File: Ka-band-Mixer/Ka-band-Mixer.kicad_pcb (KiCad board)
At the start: 4 copper layers, 58.9 x 41.9 mm, 75 parts, among them J1 Conn_01x02_Male, J2 Conn_01x02_Male, J3 Connector_Conn_01x02_Male, J4 Conn_01x05_Male, J5 SMA_END-frequencySintesizer, U1 ADF4150HV, U2 LT1962-3.3, U3 LT3010, U4 HMC739LP4E, U5 LT1962-5, U6 LT1962-5, U7 HMC292ALC3B, X1 IQXT-220-1

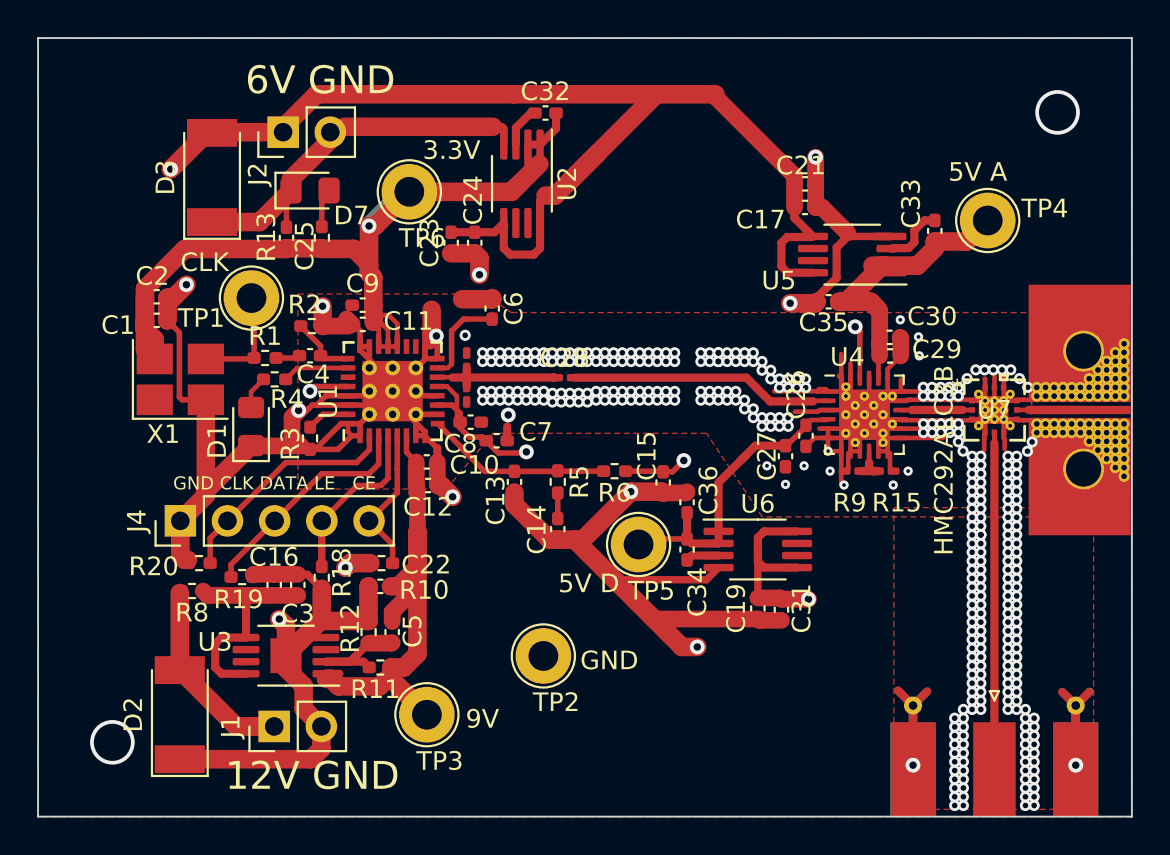
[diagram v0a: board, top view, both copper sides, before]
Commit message: update bom
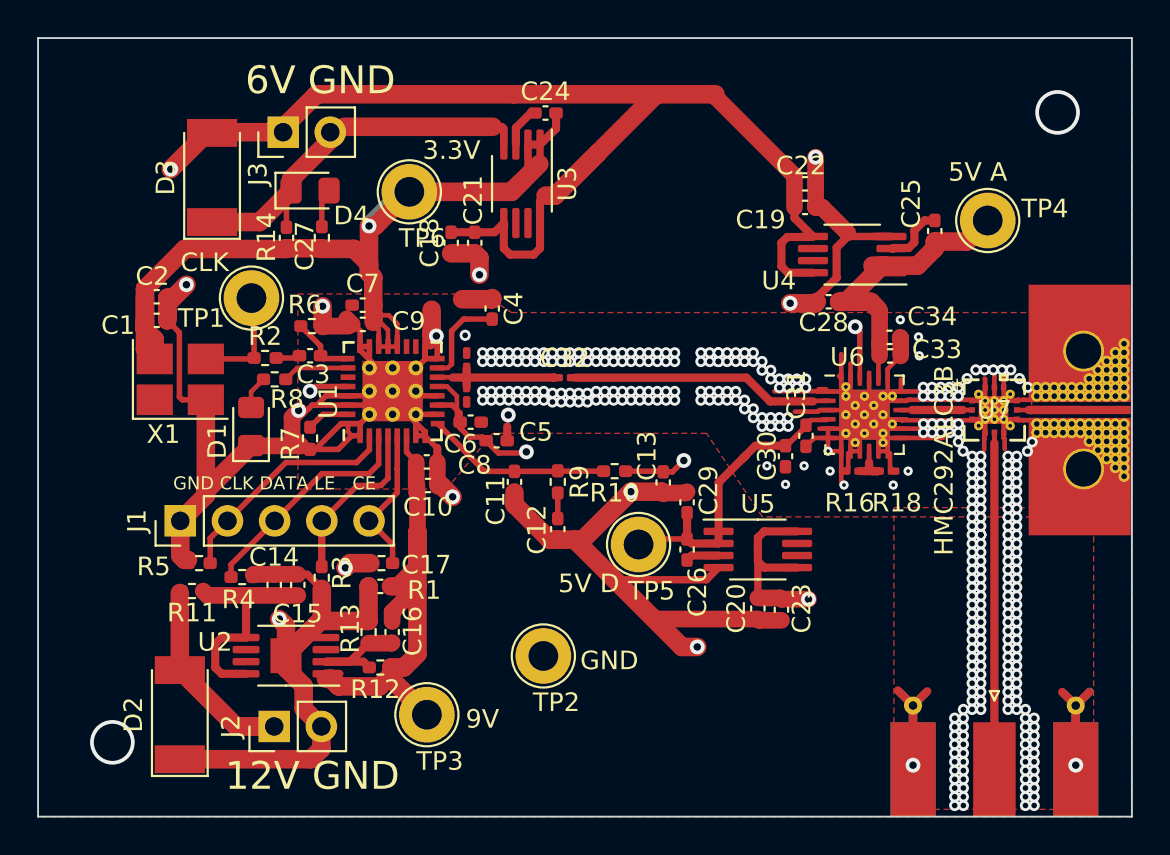
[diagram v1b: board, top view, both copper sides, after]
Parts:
- renumbered C12 to C10, C13 to C11, C14 to C12, C15 to C13, C16 to C14, C3 to C15, C5 to C16, C22 to C17, C23 to C18, C17 to C19, C19 to C20, C24 to C21, C21 to C22, C31 to C23, C32 to C24, C33 to C25, C34 to C26, C25 to C27, C35 to C28, C36 to C29, C4 to C3, C27 to C30, C26 to C31, C28 to C32, C29 to C33, C30 to C34, C6 to C4, C7 to C5, C8 to C6, C9 to C7, C10 to C8, C11 to C9, D7 to D4, J4 to J1, J1 to J2, J2 to J3, J3 to J4, R10 to R1, R6 to R10, R8 to R11, R11 to R12, R12 to R13, R13 to R14, R7 to R15, R9 to R16, R14 to R17, R15 to R18, R1 to R2, R18 to R3, R19 to R4, R20 to R5, R2 to R6, R3 to R7, R4 to R8, R5 to R9, U3 to U2, U2 to U3, U5 to U4, U6 to U5, U4 to U6
